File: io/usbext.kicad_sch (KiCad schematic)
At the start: 13 parts, among them J15 USB_A_Stacked

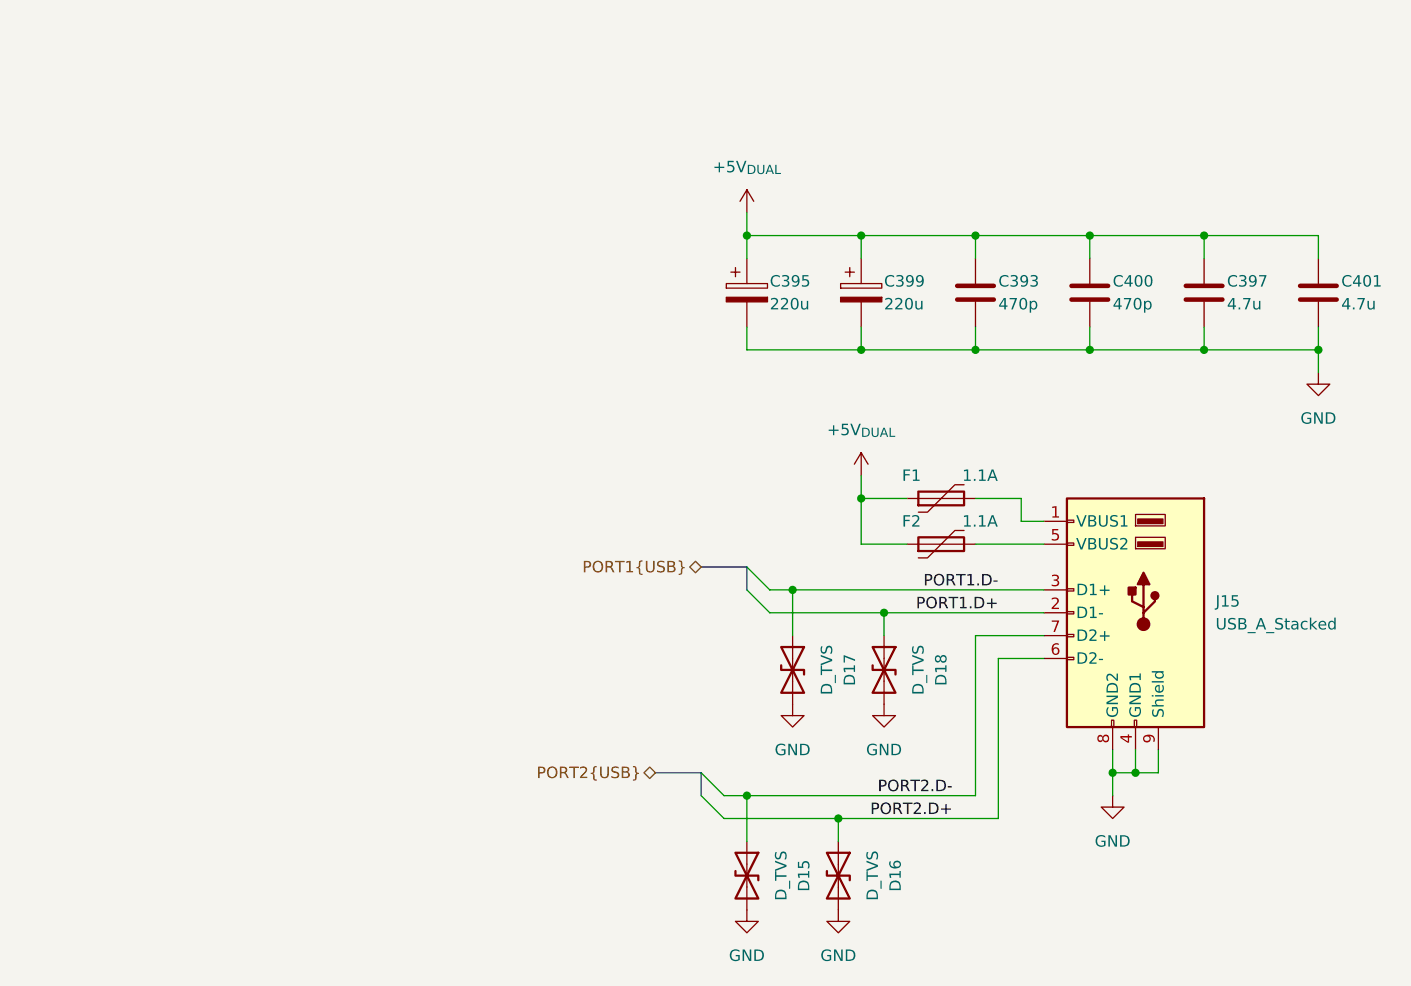
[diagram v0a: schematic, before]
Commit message: External I/O
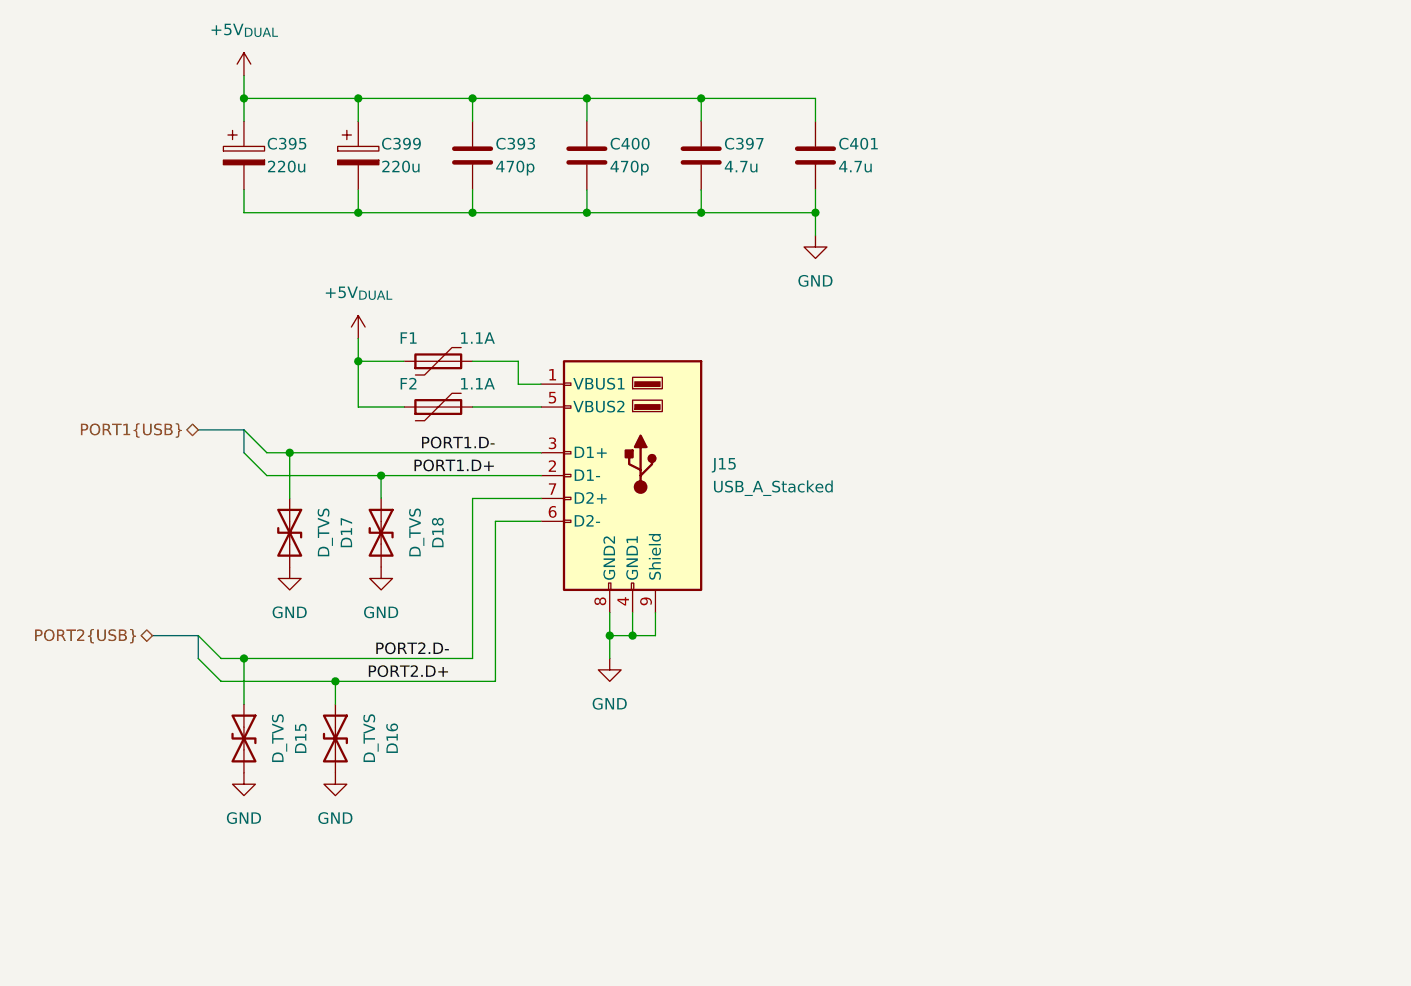
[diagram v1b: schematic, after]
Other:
- moved on the sheet: C393, C395, C397, C399, C400, C401, D15, D16, D17, D18, F1, F2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
